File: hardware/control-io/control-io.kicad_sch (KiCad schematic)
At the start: 30 parts, among them J1 3.5mm TRS MIDI IN, J2 6.35mm TRS EXPRESSION, J3 RASPBERRY PI CONTROL HEADER, SW1A DPDT POLARITY — POLE A, SW1B DPDT POLARITY — POLE B, U1 6N138, U2 ADS1115IDGS (ADDR=GND / 0x48)

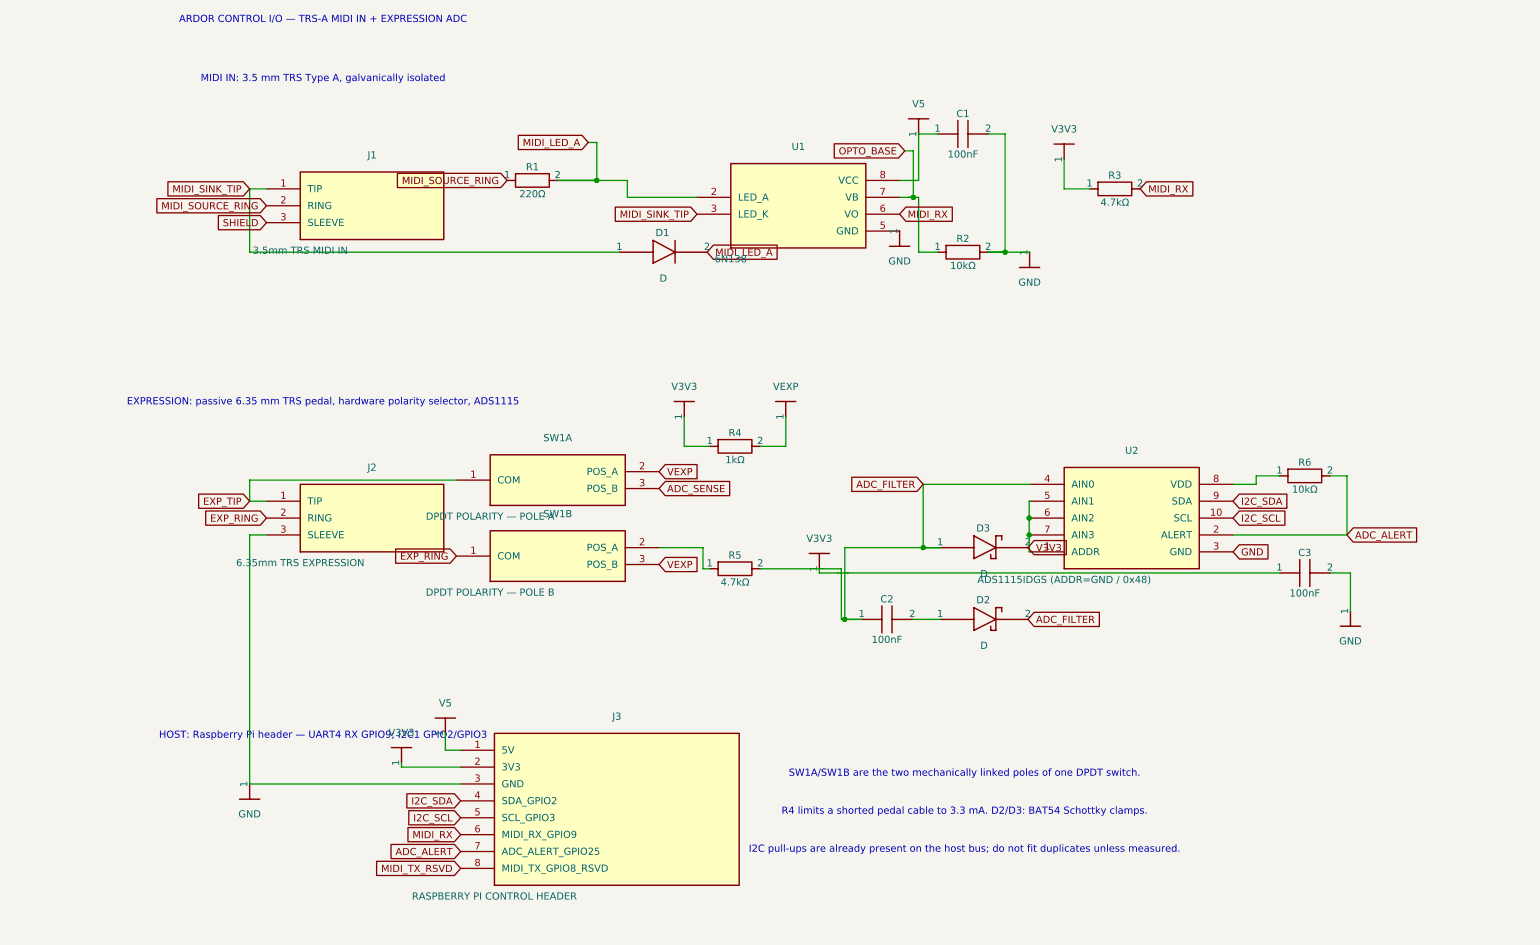
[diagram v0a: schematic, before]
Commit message: fix: code review fixes
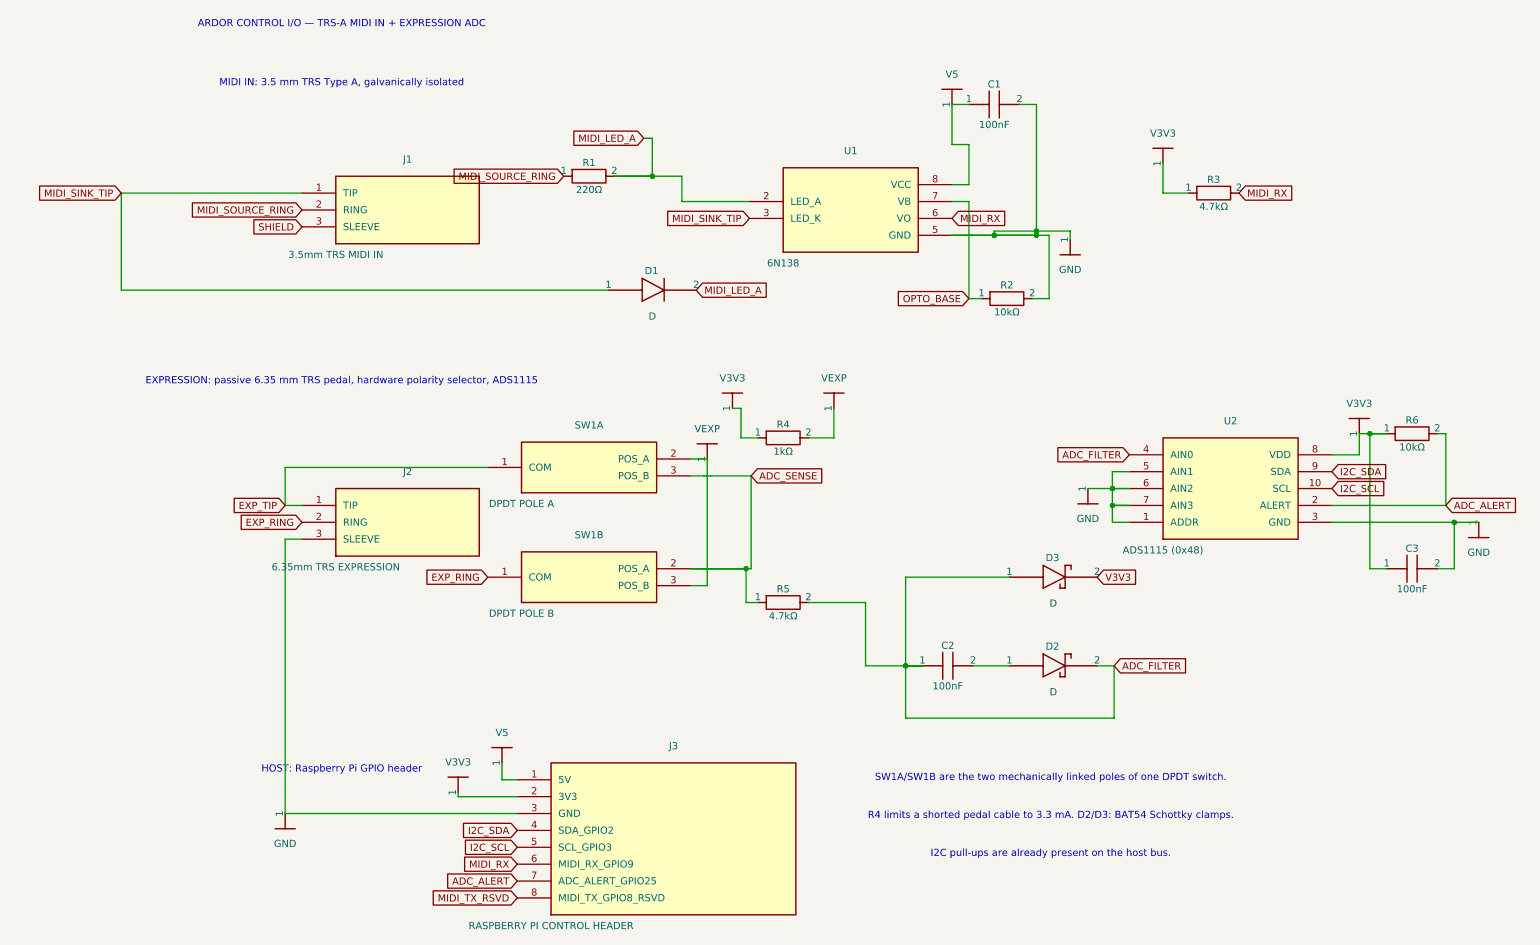
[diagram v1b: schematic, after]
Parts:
- removed GND (x4): GND, symbol Custom:rail_down
- removed SW1A: DPDT POLARITY — POLE A, symbol Device:U_DPDT_POLARITY_—_POLE_A
- removed SW1B: DPDT POLARITY — POLE B, symbol Device:U_DPDT_POLARITY_—_POLE_B
- removed U2: ADS1115IDGS (ADDR=GND / 0x48), symbol Device:U_ADS1115IDGS_(ADDR=GND_0x48)
- removed V3V3 (x4): V3V3, symbol Custom:rail_up
- removed V5 (x2): V5, symbol Custom:rail_up
- removed VEXP: VEXP, symbol Custom:rail_up
- added GND (x4): GND, symbol Custom:rail_down
- added SW1A: DPDT POLE A, symbol Device:U_DPDT_POLE_A
- added SW1B: DPDT POLE B, symbol Device:U_DPDT_POLE_B
- added U2: ADS1115 (0x48), symbol Device:U_ADS1115_(0x48)
- added V3V3 (x4): V3V3, symbol Custom:rail_up
- added V5 (x2): V5, symbol Custom:rail_up
- added VEXP (x2): VEXP, symbol Custom:rail_up
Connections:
- net ADC_ALERT: now also U2.2 (ALERT)
- net ADC_FILTER: now also U2.4 (AIN0)
- net ADC_SENSE: now also R5.1, SW1A.3 (POS_B), SW1B.2 (POS_A)
- net EXP_RING: now also SW1B.1 (COM)
- net EXP_TIP: now also SW1A.1 (COM)
- net I2C_SCL: now also U2.10 (SCL)
- net I2C_SDA: now also U2.9 (SDA)
- net at C1.1, U1.8 (VCC): now also V5.1
- net at C1.2, R2.2: now also U1.5 (GND), GND.1
- net at R4.2: now also VEXP.1
- net at J3.2 (3V3): now also V3V3.1
- net at J2.3 (SLEEVE), J3.3 (GND): now also GND.1
- net at J3.1 (5V): now also V5.1
- net at R6.1: now also C3.1, U2.8 (VDD), V3V3.1
- net at R4.1: now also V3V3.1
- net at R3.1: now also V3V3.1
- net at C3.2: now also GND.1, U2.3 (GND)
- new net: SW1A.2 (POS_A), SW1B.3 (POS_B), VEXP.1
- new net: GND.1, U2.1 (ADDR), U2.5 (AIN1), U2.6 (AIN2), U2.7 (AIN3)
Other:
- note added: "HOST: Raspberry Pi GPIO header"
- note added: "I2C pull-ups are already present on the host bus."
- note removed: "HOST: Raspberry Pi header — UART4 RX GPIO9; I2C1 GPIO2/GPIO3"
- note removed: "I2C pull-ups are already present on the host bus; do not fit duplicates unless measured."
